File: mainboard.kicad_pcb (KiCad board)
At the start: 2 copper layers, 88 x 100 mm, 57 parts, among them J1 USB_C_Receptacle_USB2.0, J2 GPIO, J3 RJ45, J4 RJ45, J5 Conn_01x02_Socket, J6 Conn_01x03_Socket, M1 Fan, Q1 MMBT3904, Q2 MMBT3906, Q3 SSM3J332R, Q4 MMBT3906, SW1 SW_DIP_x02, U1 CH221K, U2 MCP251863, U3 NJM2391, U4 MSP2807, U6 IM920sl, Y1 4MHz

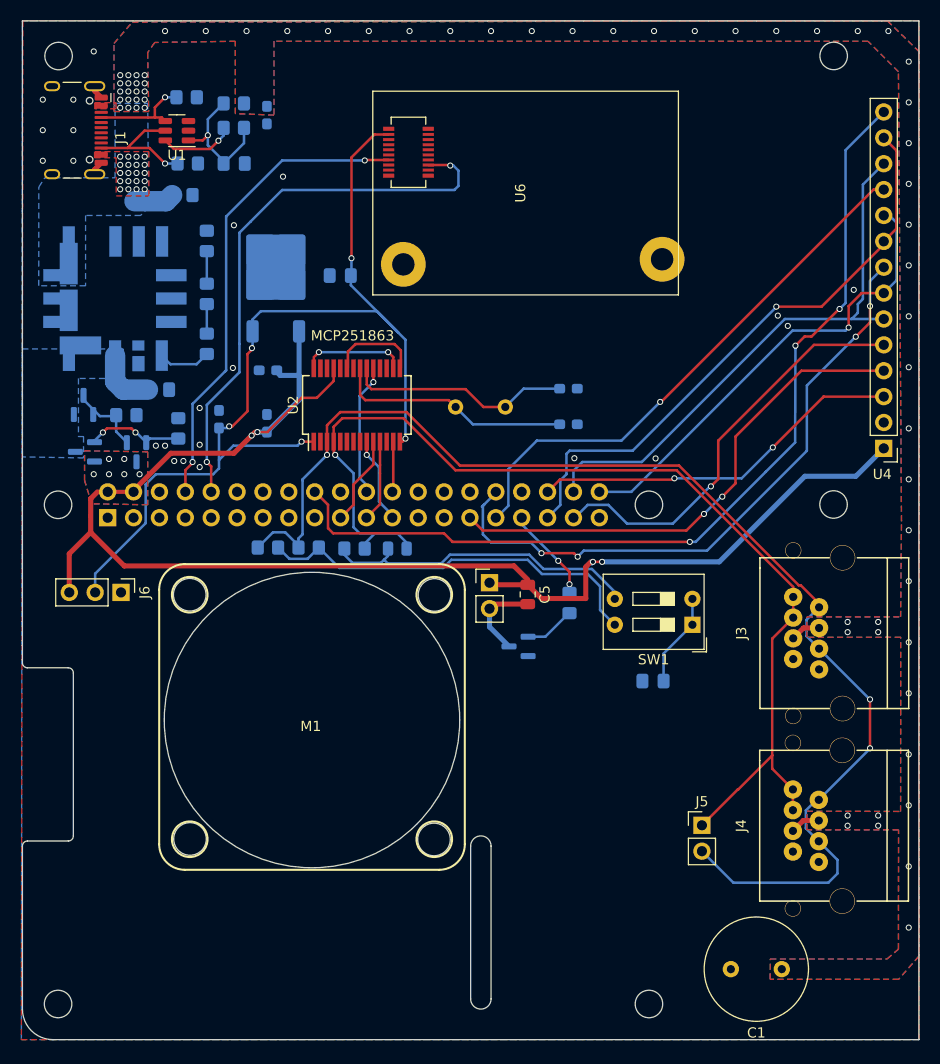
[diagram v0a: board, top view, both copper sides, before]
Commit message: first commit
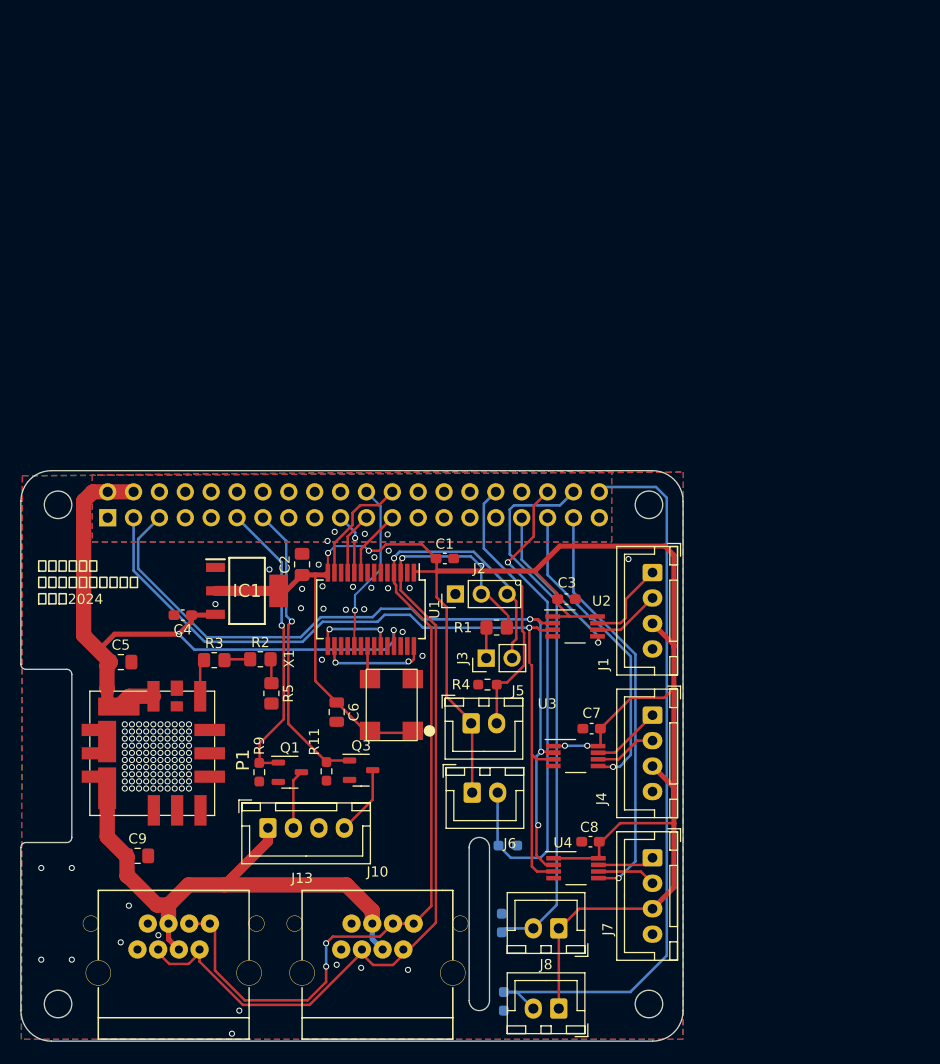
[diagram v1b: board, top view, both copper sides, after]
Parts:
- removed ? (x3): , 
- removed C10: 4700pF, Capacitor_SMD:C_0805_2012Metric_Pad1.18x1.45mm_HandSolder
- removed C11: 0.1μF, Capacitor_SMD:C_0603_1608Metric_Pad1.08x0.95mm_HandSolder
- removed C12: 10µF, Capacitor_SMD:C_0805_2012Metric_Pad1.18x1.45mm_HandSolder
- removed M1: Fan, pihat_cooling:fan_30mm
- removed Q2, Q4: MMBT3906, Package_TO_SOT_SMD:SOT-23
- removed R10: 10KΩ, Resistor_SMD:R_0805_2012Metric_Pad1.20x1.40mm_HandSolder
- removed R12, R13, R14: 120Ω, Resistor_SMD:R_0805_2012Metric_Pad1.20x1.40mm_HandSolder
- removed R15: 120Ω, Resistor_SMD:R_0805_2012Metric
- removed S1, S2, S3, S4: M3, screw:M3
- removed SW1: SW_DIP_x02, Button_Switch_THT:SW_DIP_SPSTx02_Slide_9.78x7.26mm_W7.62mm_P2.54mm
- removed U6: IM920sl, interplan:IM920s
- removed Y1: 4MHz, Crystal:Crystal_HC49-U_Vertical
- added IC1: AZ1117CH-3.3TRG1, OKL:SOT230P700X180-4N, F.Cu at (130.2, 109.8)
- added J10: RJ45, OKL:7810-8P8C, F.Cu at (143.0, 145.0)
- added J11: Conn_01x02, Connector_JST:JST_XH_B2B-XH-A_1x02_P2.50mm_Vertical, F.Cu at (160.8, 150.8)
- added J13: Conn_01x04_Socket, Connector_JST:JST_XH_B4B-XH-A_1x04_P2.50mm_Vertical, F.Cu at (132.2, 133.1)
- added J2: Conn_01x03_Socket, Connector_PinHeader_2.54mm:PinHeader_1x03_P2.54mm_Vertical, F.Cu at (150.7, 110.1)
- added J7: Conn_01x04, Connector_JST:JST_XH_B4B-XH-A_1x04_P2.50mm_Vertical, F.Cu at (170.0, 136.0)
- added J8: Conn_01x02, Connector_JST:JST_XH_B2B-XH-A_1x02_P2.50mm_Vertical, F.Cu at (160.8, 142.9)
- added J9: RJ45, OKL:7810-8P8C, F.Cu at (123.0, 145.0)
- added X1: CSX-750P, OKL:CSX-750P, F.Cu at (144.4, 121.0)
- C1: value 1000μF -> 0.1μF; footprint Capacitor_THT:C_Radial_D10.0mm_H12.5mm_P5.00mm -> Capacitor_SMD:C_0603_1608Metric_Pad1.08x0.95mm_HandSolder
- C2: value 1μF -> 10µF; moved to F.Cu
- C3, C7: moved to F.Cu
- C4: value 10μF -> 0.1μF; footprint Capacitor_SMD:C_0805_2012Metric_Pad1.18x1.45mm_HandSolder -> Capacitor_SMD:C_0603_1608Metric_Pad1.08x0.95mm_HandSolder; moved to F.Cu
- C5: value 100nF -> 10μF; footprint Capacitor_SMD:C_0805_2012Metric -> Capacitor_SMD:C_0805_2012Metric_Pad1.18x1.45mm_HandSolder
- C6: value 0.1μF -> 100nF; footprint Capacitor_SMD:C_0603_1608Metric_Pad1.08x0.95mm_HandSolder -> Capacitor_SMD:C_0805_2012Metric; moved to F.Cu
- C8: value 22pF -> 0.1μF; moved to F.Cu
- C9: value 22pF -> 22μF; footprint Capacitor_SMD:C_0603_1608Metric_Pad1.08x0.95mm_HandSolder -> Capacitor_SMD:C_0805_2012Metric_Pad1.18x1.45mm_HandSolder; moved to F.Cu
- J1: value USB_C_Receptacle_USB2.0 -> Conn_01x04; footprint Connector_USB:USB_C_Receptacle_HCTL_HC-TYPE-C-16P-01A -> Connector_JST:JST_XH_B4B-XH-A_1x04_P2.50mm_Vertical
- J3: value RJ45 -> Conn_01x02_Socket; footprint akiRJ45:7810-8P8C -> Connector_PinHeader_2.54mm:PinHeader_1x02_P2.54mm_Vertical
- J4: value RJ45 -> Conn_01x04; footprint akiRJ45:7810-8P8C -> Connector_JST:JST_XH_B4B-XH-A_1x04_P2.50mm_Vertical
- J5: value Conn_01x02_Socket -> Conn_01x02; footprint Connector_PinHeader_2.54mm:PinHeader_1x02_P2.54mm_Vertical -> Connector_JST:JST_XH_B2B-XH-A_1x02_P2.50mm_Vertical
- J6: value Conn_01x03_Socket -> Conn_01x02; footprint Connector_PinHeader_2.54mm:PinHeader_1x03_P2.54mm_Vertical -> Connector_JST:JST_XH_B2B-XH-A_1x02_P2.50mm_Vertical
- P1: value ~ -> OKLT6W12NC; footprint okL:OKLT6W12NC -> OKL:OKLT6W12NC; moved to F.Cu
- Q1: value MMBT3904 -> IRFML8244TRPBF; footprint Package_TO_SOT_SMD:SOT-23 -> Package_TO_SOT_SMD:SOT-23-3; moved to F.Cu
- Q3: value SSM3J332R -> IRFML8244TRPBF; footprint Package_TO_SOT_SMD:SOT-23 -> Package_TO_SOT_SMD:SOT-23-3; moved to F.Cu
- R1: value 1kΩ -> 120Ω; moved to F.Cu
- R11: value 10KΩ -> R; footprint Resistor_SMD:R_0805_2012Metric_Pad1.20x1.40mm_HandSolder -> Resistor_SMD:R_0603_1608Metric_Pad0.98x0.95mm_HandSolder; moved to F.Cu
- R2: value 5.1kΩ -> 330Ω; moved to F.Cu
- R3: value 5.1kΩ -> 1kΩ; moved to F.Cu
- R4: value 47kΩ -> R; footprint Resistor_SMD:R_0805_2012Metric_Pad1.20x1.40mm_HandSolder -> Resistor_SMD:R_0603_1608Metric_Pad0.98x0.95mm_HandSolder; moved to F.Cu
- R5: value 20KΩ -> 10Ω; moved to F.Cu
- R6: value 100 -> R; footprint Resistor_SMD:R_0805_2012Metric_Pad1.20x1.40mm_HandSolder -> Resistor_SMD:R_0603_1608Metric_Pad0.98x0.95mm_HandSolder
- R7: value 1kΩ -> R; footprint Resistor_SMD:R_0805_2012Metric_Pad1.20x1.40mm_HandSolder -> Resistor_SMD:R_0603_1608Metric_Pad0.98x0.95mm_HandSolder
- R8: value 330Ω -> R; footprint Resistor_SMD:R_0805_2012Metric_Pad1.20x1.40mm_HandSolder -> Resistor_SMD:R_0603_1608Metric_Pad0.98x0.95mm_HandSolder
- R9: value 10Ω -> R; footprint Resistor_SMD:R_0805_2012Metric_Pad1.20x1.40mm_HandSolder -> Resistor_SMD:R_0603_1608Metric_Pad0.98x0.95mm_HandSolder; moved to F.Cu
- U1: value CH221K -> MCP251863; footprint Package_TO_SOT_SMD:SOT-23-6 -> Package_SO:SSOP-28_5.3x10.2mm_P0.65mm
- U2: value MCP251863 -> TCA9803; footprint Package_SO:SSOP-28_5.3x10.2mm_P0.65mm -> Package_SO:VSSOP-8_3.0x3.0mm_P0.65mm
- U3: value NJM2391 -> TCA9803; footprint Package_TO_SOT_SMD:TO-252-2 -> Package_SO:VSSOP-8_3.0x3.0mm_P0.65mm; moved to F.Cu
- U4: value MSP2807 -> TCA9803; footprint MSP2807:MSP2807 -> Package_SO:VSSOP-8_3.0x3.0mm_P0.65mm
- moved R8 75.3 mm to (155.4, 150.1), turned to -90 degrees
- moved J1 72.3 mm to (170.0, 108.0)
- moved R7 63.8 mm to (155.2, 142.4)
- moved C9 62.4 mm to (119.5, 135.8), turned to 0 degrees
- moved R4 60.1 mm to (153.8, 119.0)
- moved R1 57.6 mm to (154.7, 113.4), turned to 0 degrees
- moved P1 57.0 mm to (114.8, 131.8), turned to 90 degrees
- moved C3 55.9 mm to (161.6, 110.6), turned to 0 degrees
- moved R2 55.6 mm to (131.5, 116.5)
- moved U3 55.2 mm to (162.5, 126.0), turned to 0 degrees
- moved R9 52.4 mm to (131.4, 127.6)
- moved C1 52.1 mm to (149.6, 106.6), turned to 0 degrees
- moved U1 50.7 mm to (142.4, 111.6), turned to -90 degrees
- moved R5 49.7 mm to (132.6, 119.9), turned to -90 degrees
- moved R3 48.8 mm to (127.0, 116.6)
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- renumbered J2 to J12
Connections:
- net D/C renamed EN_3
- C1 pad 1: +12V -> +3.3V
- C2 pad 1: Net-(U1-VDD) -> +3.3V
- C3 pad 1: +12V -> +3.3V
- C4 pad 1: Net-(P1-Sence) -> +5V
- C5 pad 2: Net-(M1--) -> GND
- C7 pad 1: +5V -> +3.3V
- C8 pad 1: GND -> +3.3V
- C8 pad 2: Net-(U2-OSC1) -> GND
- C9 pad 1: GND -> +12V
- C9 pad 2: Net-(U2-OSC2) -> GND
- J12 pad 11: /GPIO17 -> LED_B
- J12 pad 13: /GPIO27 -> LED_R
- J12 pad 32: LED -> limit1
- J12 pad 33: GPIO13/PWM1 -> EN_1
- J12 pad 35: SPI1.MISO -> EN_2
- J12 pad 36: SPI1.CE0 -> limit2
- J12 pad 38: SPI1.MOSI -> limit3
- J12 pad 40: SPI1.SCLK -> limit4
- J3 pad 1: /canfd/CANH -> Net-(J3-Pin_1)
- J3 pad 2: /canfd/CANL -> /canfd/CANH
- J4 pad 1: /canfd/CANH -> Net-(J4-Pin_1)
- J4 pad 2: /canfd/CANL -> Net-(J4-Pin_2)
- J4 pad 3: /canfd/CANH -> +3.3V
- J4 pad 4: +12V -> GND
- J5 pad 1: /canfd/CANH -> +3.3V
- J5 pad 2: /canfd/CANL -> limit1
- J6 pad 1: GND -> +3.3V
- J6 pad 2: +3.3V -> limit2
- P1 pad 4: Net-(P1-Sence) -> +5V
- P1 pad 5: Net-(P1-Sence) -> +5V
- Q1 pad 1: Net-(Q1-B) -> LED_B
- Q1 pad 3: Net-(M1--) -> Net-(J13-Pin_2)
- Q3 pad 1: Net-(Q3-G) -> LED_R
- Q3 pad 2: +5V -> GND
- Q3 pad 3: Net-(P1-Sence) -> Net-(J13-Pin_4)
- R1 pad 1: +12V -> Net-(J3-Pin_1)
- R1 pad 2: Net-(U1-VDD) -> /canfd/CANL
- R11 pad 1: Net-(Q3-G) -> GND
- R11 pad 2: GND -> LED_R
- R2 pad 1: Net-(J1-CC1) -> Net-(R2-Pad1)
- R2 pad 2: GND -> Net-(R2-Pad2)
- R3 pad 1: Net-(J1-CC2) -> Net-(P1-Trim)
- R3 pad 2: GND -> Net-(R2-Pad1)
- R4 pad 1: Net-(U1-VDD) -> limit1
- R4 pad 2: Net-(U1-CFG) -> GND
- R5 pad 1: +12V -> Net-(R2-Pad2)
- R6 pad 1: Net-(Q1-B) -> limit2
- R6 pad 2: GPIO13/PWM1 -> GND
- R7 pad 1: Net-(P1-Trim) -> limit3
- R7 pad 2: Net-(R7-Pad2) -> GND
- R8 pad 1: Net-(R7-Pad2) -> limit4
- R8 pad 2: Net-(R8-Pad2) -> GND
- R9 pad 1: Net-(R8-Pad2) -> GND
- R9 pad 2: GND -> LED_B
- U1 pad 1: Net-(U1-VDD) -> +3.3V
- U1 pad 2: GND -> unconnected-(U1-NC-Pad2)
- U1 pad 3: unconnected-(U1-PG-Pad3) -> /canfd/CANL
- U1 pad 4: Net-(J1-CC1) -> /canfd/CANH
- U1 pad 5: Net-(J1-CC2) -> GND
- U1 pad 6: Net-(U1-CFG) -> unconnected-(U1-nINT1-Pad6)
- U2 pad 2: unconnected-(U2-NC-Pad2) -> /GPIO3/SCL1
- U2 pad 3: /canfd/CANL -> /GPIO2/SDA1
- U2 pad 4: /canfd/CANH -> GND
- U2 pad 5: GND -> EN_1
- U2 pad 6: unconnected-(U2-nINT1-Pad6) -> Net-(J1-Pin_2)
- U2 pad 7: unconnected-(U2-nINT0-Pad7) -> Net-(J1-Pin_1)
- U2 pad 8: unconnected-(U2-NC-Pad8) -> +3.3V
- U3 pad 1: +5V -> +3.3V
- U3 pad 2: GND -> /GPIO3/SCL1
- U3 pad 3: +3.3V -> /GPIO2/SDA1
- U4 pad 1: +5V -> +3.3V
- U4 pad 2: GND -> /GPIO3/SCL1
- U4 pad 3: SPI1.CE0 -> /GPIO2/SDA1
- U4 pad 4: RESET -> GND
- U4 pad 6: SPI1.MOSI -> Net-(J7-Pin_2)
- U4 pad 7: SPI1.SCLK -> Net-(J7-Pin_1)
- U4 pad 8: LED -> +3.3V
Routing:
- net +3.3V: track 98.5 -> 198.8 mm, vias 5 -> 4
- net IRQ: track 91.4 -> 0.00 mm, vias 3 -> 0
- net +5V: track 147.0 -> 66.8 mm, vias 10 -> 2
- net /GPIO3/SCL1: track 0.00 -> 79.5 mm, vias 0 -> 3
- net /GPIO2/SDA1: track 0.00 -> 79.4 mm, vias 0 -> 1
- net limit4: track 0.00 -> 73.3 mm
- net LED: track 63.2 -> 0.00 mm, vias 4 -> 0
- net SPI1.MISO: track 58.4 -> 0.00 mm, vias 1 -> 0
- net SPI1.MOSI: track 55.2 -> 0.00 mm
- net UART RXD: track 55.1 -> 0.00 mm, vias 2 -> 0
- net limit3: track 0.00 -> 54.2 mm
- net SPI1.CE1: track 53.5 -> 0.06 mm, vias 1 -> 0
- net RESET: track 50.7 -> 0.00 mm, vias 2 -> 0
- net limit2: track 0.00 -> 49.4 mm, vias 0 -> 1
- net UART TXD: track 47.0 -> 0.00 mm, vias 2 -> 0
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- removed copper zone on B.Cu, net +12V
- removed copper zone on F.Cu, net +12V
- removed copper zone on B.Cu, net +5V
- removed copper zone on F.Cu, net +5V
- removed copper zone on B.Cu, net Net-(P1-Sence)
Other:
- board size 88 x 100 mm -> 65 x 56 mm
- board text added: "サレジオ高専 ロボコンプロジェクト 制御班2024"
- board text removed: "PoE"
